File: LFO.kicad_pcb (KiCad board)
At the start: 2 copper layers, 39.6 x 100 mm, 98 parts, among them J1 AudioJack2_SwitchT, J2 AudioJack2_SwitchT, J3 AudioJack2_SwitchT, J4 AudioJack2_SwitchT, J5 AudioJack2_SwitchT, J6 AudioJack2_SwitchT, J7 Conn_02x03_Odd_Even, J8 Conn_02x05_Odd_Even, Q1 BC847, SW1 SW_Push, SW2 SW_SPDT_MSM, SW3 SW_SPDT_MSM, U1 ATtiny84-20MU, U2 74AHCT1G125, U3 MCP6002-xMS, U4 MCP6002-xMS, U5 L7805, U6 LM324, Y1 20MHz

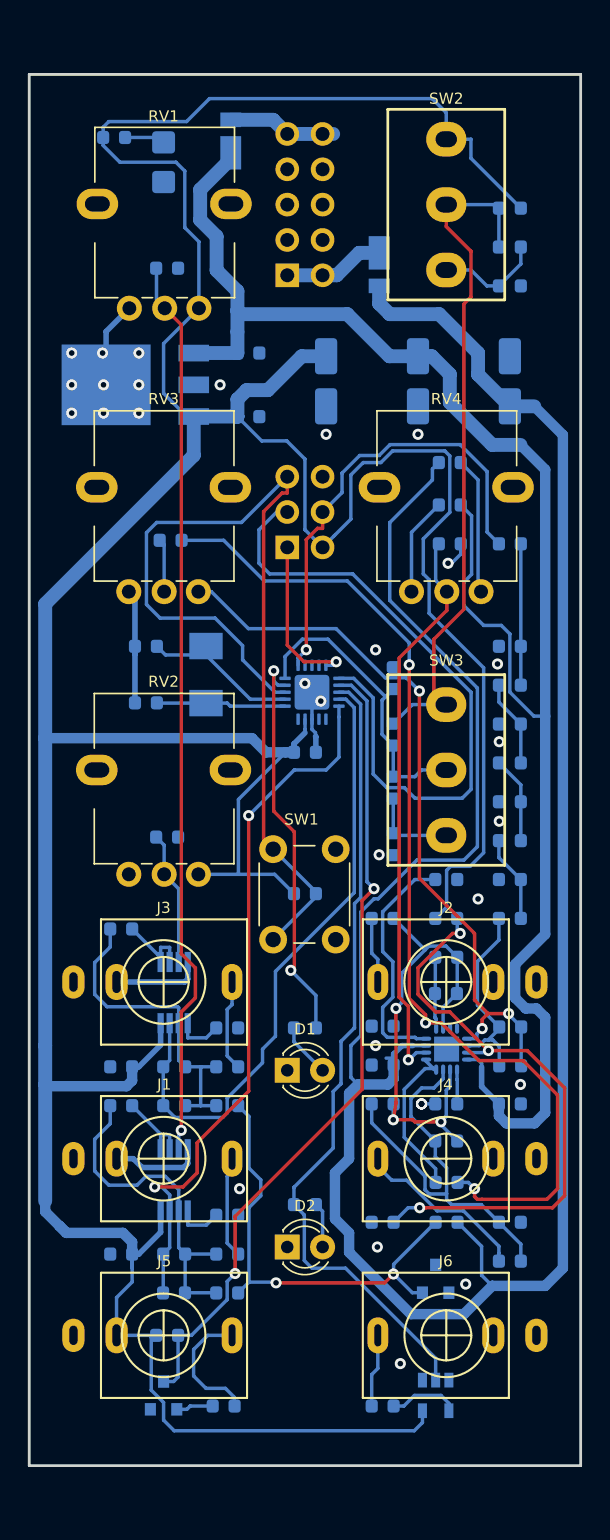
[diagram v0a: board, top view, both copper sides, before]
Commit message: Initial placement and power.
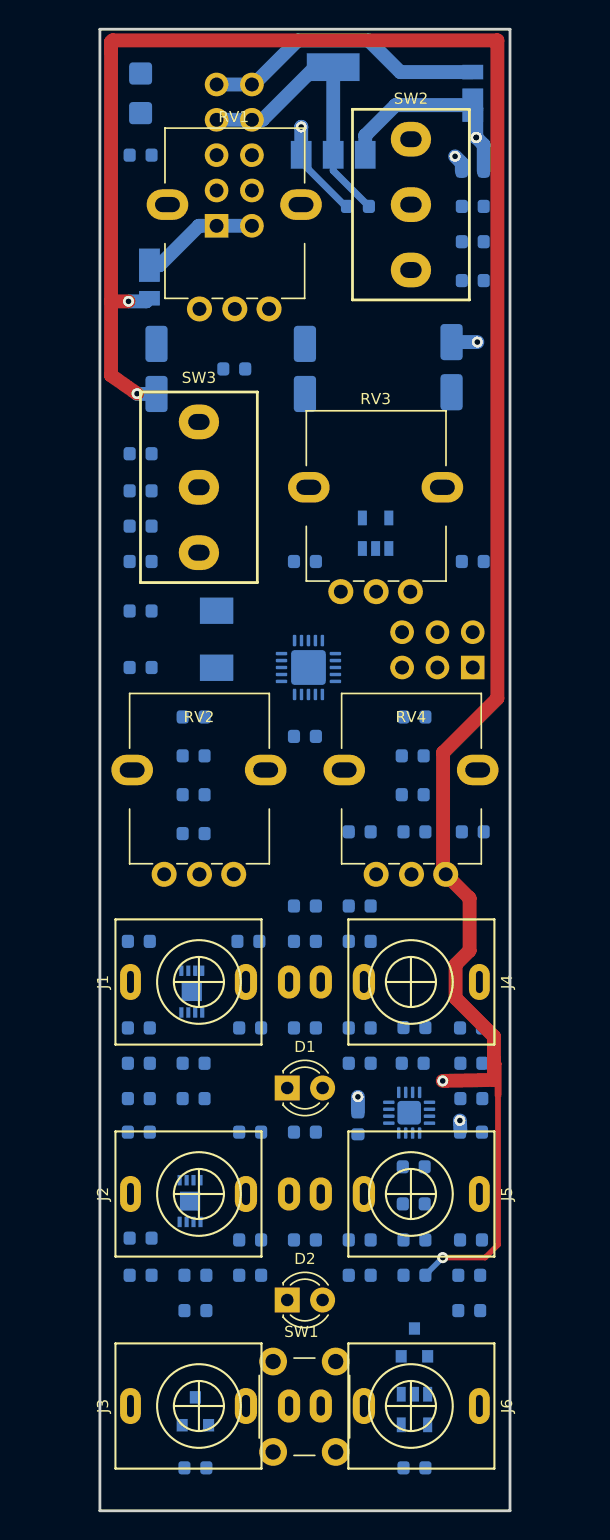
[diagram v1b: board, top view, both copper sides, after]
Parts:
- added R45: 100k, Resistor_SMD:R_0603_1608Metric, B.Cu at (152.4, 141.3)
- added R46: 220k, Resistor_SMD:R_0603_1608Metric, B.Cu at (152.4, 123.5)
- added R47: 220k, Resistor_SMD:R_0603_1608Metric, B.Cu at (152.4, 126.1)
- added U7: 74AHCT1G125, Package_TO_SOT_SMD:SOT-23-5, B.Cu at (153.6, 88.0)
- R19, R25, R31, R32, R33: value 68k -> 100k
- R28, R36: value 33k -> 47k
- R37: value 68k -> 47k
- RV2, RV4: footprint Local:AlpsRK09K -> Local:R09M3KT
- U3, U4: footprint Package_SO:MSOP-8_3x3mm_P0.65mm -> Package_DFN_QFN:DFN-8-1EP_3x2mm_P0.5mm_EP1.36x1.46mm
- U5: footprint Package_TO_SOT_SMD:TO-252-3_TabPin2 -> Package_TO_SOT_SMD:SOT-223-3_TabPin2
- U6: value LM324 -> LM324QT; footprint Package_DFN_QFN:QFN-16-1EP_3x3mm_P0.5mm_EP1.8x1.8mm -> Package_DFN_QFN:QFN-16-1EP_3x3mm_P0.5mm_EP1.7x1.7mm
- moved R32 53.2 mm to (152.4, 138.8), turned to 180 degrees
- moved R37 49.2 mm to (148.5, 131.0)
- moved SW1 36.8 mm to (146.2, 154.0)
- moved J3 30.6 mm to (140.9, 150.7), turned to 90 degrees
- moved R43 27.3 mm to (136.7, 90.0), turned to 180 degrees
- moved SW3 27.0 mm to (140.9, 84.7)
- moved R1 26.8 mm to (160.6, 90.0), turned to 180 degrees
- moved R41 26.1 mm to (136.7, 87.5), turned to 0 degrees
- moved C14 25.4 mm to (137.8, 76.2)
- moved R39 25.2 mm to (136.7, 84.9), turned to 180 degrees
- moved R25 25.0 mm to (152.4, 109.4), turned to 180 degrees
- moved C25 24.3 mm to (136.7, 82.3), turned to 0 degrees
- moved U5 24.3 mm to (150.5, 57.6), turned to 90 degrees
- moved J2 23.4 mm to (140.9, 135.5)
- moved R30 23.4 mm to (148.5, 114.8)
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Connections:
- C21 pad 2: Net-(C16-Pad1) -> Net-(C21-Pad2)
- J2 pad T: /OutputStage/Out -> /CVIn05.sch/In
- J2 pad TN: Net-(J2-PadTN) -> GND
- J3 pad T: /CVIn05.sch/In -> /DigitalIn/In
- J3 pad TN: GND -> +5V
- J4 pad T: /OutputStage/Inv -> /OutputStage/Out
- J5 pad T: /DigitalIn/In -> /OutputStage/Inv
- J5 pad TN: +5V -> Net-(J5-PadTN)
- J7 pad 1: MISO -> LED1
- R19 pad 1: Net-(C16-Pad1) -> /OutputStage/Out
- R20 pad 2: MOSI -> OUT
- R31 pad 1: Net-(C21-Pad1) -> /OutputStage/Inv
- R31 pad 2: Net-(C16-Pad1) -> Net-(C21-Pad2)
- R32 pad 2: +12V -> Net-(R25-Pad1)
- R33 pad 2: Net-(C16-Pad2) -> Net-(C21-Pad2)
- R37 pad 1: -12V -> GND
- R6 pad 1: TRIG -> LED2
- RV4 pad 1: Net-(R37-Pad2) -> -12V
- RV4 pad 3: Net-(R32-Pad1) -> +12V
- U1 pad 14: LED1 -> LED2
- U1 pad 20: MISO -> LED1
- U6 pad 1: Net-(C15-Pad1) -> Net-(R29-Pad1)
- U6 pad 10: Net-(C22-Pad1) -> (no net)
- U6 pad 15: (no net) -> Net-(C15-Pad1)
- U6 pad 16: (no net) -> Net-(C15-Pad2)
- U6 pad 2: Net-(C15-Pad2) -> +12V
- U6 pad 3: Net-(R29-Pad1) -> (no net)
- U6 pad 4: +12V -> Net-(R36-Pad2)
- U6 pad 5: Net-(R36-Pad2) -> Net-(C21-Pad2)
- U6 pad 6: Net-(C16-Pad1) -> Net-(C21-Pad1)
- U6 pad 7: Net-(C21-Pad1) -> Net-(R33-Pad1)
- U6 pad 8: Net-(R33-Pad1) -> Net-(R32-Pad1)
- U6 pad 9: Net-(R33-Pad1) -> Net-(R37-Pad2)
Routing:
- net +5V: track 303.7 -> 7.15 mm, vias 0 -> 1
- net Net-(C16-Pad2): track 79.9 -> 0.00 mm, vias 3 -> 0
- net RESET: track 67.1 -> 0.00 mm
- net Net-(C5-Pad1): track 65.0 -> 0.00 mm, vias 1 -> 0
- net SYNC: track 58.9 -> 0.00 mm, vias 2 -> 0
- net TRIG: track 58.1 -> 0.00 mm
- net Net-(C15-Pad1): track 52.5 -> 0.00 mm, vias 3 -> 0
- net FREQ: track 51.1 -> 0.00 mm, vias 2 -> 0
- net Net-(R38-Pad2): track 49.2 -> 0.00 mm
- net SCK: track 47.6 -> 0.00 mm
- net PWM: track 45.5 -> 0.00 mm
- net Net-(R29-Pad1): track 43.3 -> 0.00 mm, vias 3 -> 0
- net Net-(C22-Pad1): track 40.7 -> 0.00 mm, vias 1 -> 0
- net Net-(C16-Pad1): track 36.5 -> 0.00 mm, vias 3 -> 0
- net VRef-10: track 33.1 -> 0.00 mm, vias 2 -> 0
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- added copper zone on In1.Cu, net +5V
- added copper zone on In2.Cu, net GND
- removed copper zone on B.Cu, net GND
- removed copper zone on F.Cu, net GND
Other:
- board size 39.6 x 100 mm -> 29.5 x 106.5 mm
- copper layers 2 -> 4
- board text added: "Marangisto 2018, 2019"
- board text added: "Rev B"
- board text removed: "Marangisto 2018"
- board text removed: "Rev A"
